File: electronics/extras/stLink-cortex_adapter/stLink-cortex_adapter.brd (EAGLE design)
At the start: 11.4 x 20.3 mm, 2 parts, among them J15 Cortex Debug

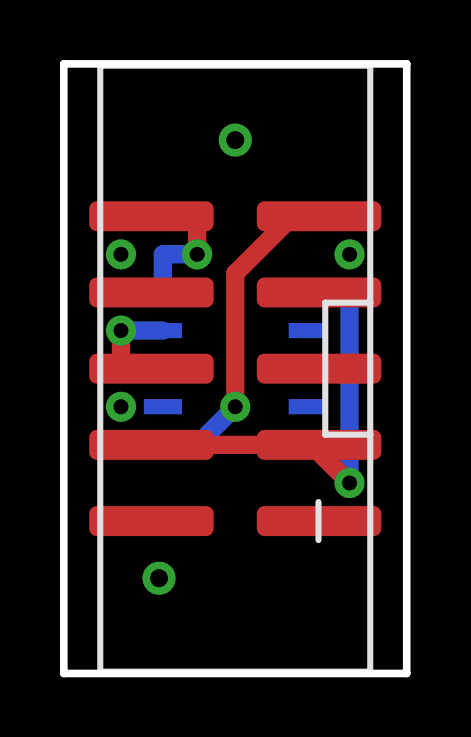
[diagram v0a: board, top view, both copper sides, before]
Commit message: Labwiz T420 module gerbers generated.
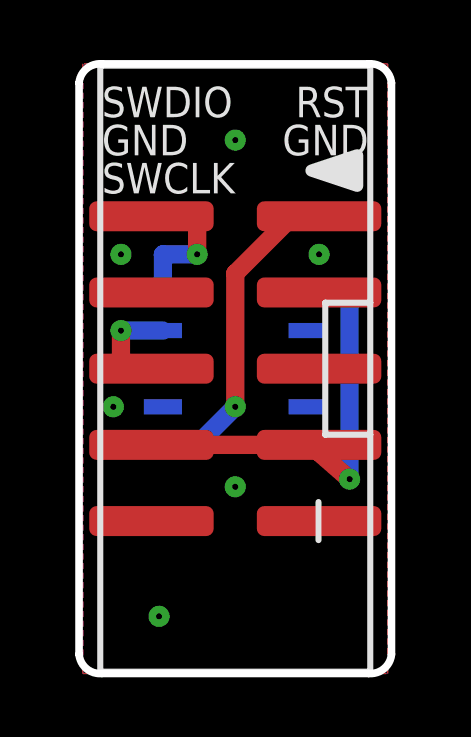
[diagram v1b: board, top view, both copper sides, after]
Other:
- board size 11.4 x 20.3 mm -> 10.4 x 20.3 mm
- board text added: "ST-Linkv2 Cortex"
- board text removed: "ST-Link v2 Cortex Adapter"
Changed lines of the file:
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@@
 <setting verticaltext="up"/>
 </settings>
-<grid distance="0.025" unitdist="inch" unit="inch" style="lines" multiple="1" display="yes" altdistance="0.05" altunitdist="mil" altunit="inch"/>
+<grid distance="5" unitdist="mil" unit="mil" style="lines" multiple="1" display="yes" altdistance="0.05" altunitdist="mil" altunit="inch"/>
 <layers>
 <layer number="1" name="Top" color="4" fill="1" visible="yes" active="yes"/>
@@
 <layer number="49" name="Reference" color="7" fill="1" visible="yes" active="yes"/>
 <layer number="50" name="dxf" color="7" fill="1" visible="no" active="no"/>
-<layer number="51" name="tDocu" color="6" fill="1" visible="yes" active="yes"/>
-<layer number="52" name="bDocu" color="7" fill="1" visible="yes" active="yes"/>
+<layer number="51" name="tDocu" color="6" fill="1" visible="no" active="yes"/>
+<layer number="52" name="bDocu" color="7" fill="1" visible="no" active="yes"/>
 <layer number="53" name="tGND_GNDA" color="7" fill="9" visible="no" active="no"/>
 <layer number="54" name="bGND_GNDA" color="1" fill="9" visible="no" active="no"/>
@@
 <board>
 <plain>
-<wire x1="-0.635" y1="0" x2="-0.635" y2="20.32" width="0.254" layer="20"/>
-<wire x1="-0.635" y1="20.32" x2="10.795" y2="20.32" width="0.254" layer="20"/>
-<wire x1="10.795" y1="20.32" x2="10.795" y2="0" width="0.254" layer="20"/>
-<wire x1="10.795" y1="0" x2="-0.635" y2="0" width="0.254" layer="20"/>
+<wire x1="9.525" y1="0" x2="0.635" y2="0" width="0.254" layer="20"/>
+<wire x1="0.635" y1="0" x2="-0.127" y2="0.635" width="0.254" layer="20" curve="-90"/>
+<wire x1="-0.127" y1="0.635" x2="-0.127" y2="19.685" width="0.254" layer="20"/>
+<wire x1="-0.127" y1="19.685" x2="0.635" y2="20.32" width="0.254" layer="20" curve="-90"/>
+<wire x1="0.635" y1="20.32" x2="9.525" y2="20.32" width="0.254" layer="20"/>
+<wire x1="9.525" y1="20.32" x2="10.287" y2="19.685" width="0.254" layer="20" curve="-90"/>
+<wire x1="10.287" y1="19.685" x2="10.287" y2="0.635" width="0.254" layer="20"/>
+<wire x1="10.287" y1="0.635" x2="9.525" y2="0" width="0.254" layer="20" curve="-90"/>
 <text x="10.16" y="15.24" size="1.016" layer="51" align="center-left">RST</text>
 <text x="0" y="12.7" size="1.016" layer="51" rot="R180" align="center-left">GND</text>
@@
 <text x="0" y="7.62" size="1.016" layer="51" rot="R180" align="center-left">3.3V</text>
 <text x="10.16" y="7.62" size="1.016" layer="51" align="center-left">3.3V</text>
-<text x="0.635" y="19.05" size="1.016" layer="22" rot="MR180" align="center-left">SWDIO</text>
-<text x="0.635" y="17.78" size="1.016" layer="22" rot="MR180" align="center-left">GND</text>
-<text x="0.635" y="16.51" size="1.016" layer="22" rot="MR180" align="center-left">SWCLK</text>
-<text x="0.635" y="15.24" size="1.016" layer="22" rot="MR180" align="center-left">3.3V</text>
-<text x="9.525" y="19.05" size="1.016" layer="22" rot="MR0" align="center-left">RST</text>
-<text x="9.525" y="15.24" size="1.016" layer="22" rot="MR0" align="center-left">3.3V</text>
-<text x="9.525" y="17.78" size="1.016" layer="22" rot="MR0" align="center-left">GND</text>
-<text x="9.525" y="6.35" size="1.4224" layer="22" rot="MR0" align="top-left">ST-Link v2
-Cortex
-Adapter</text>
+<text x="0.635" y="19.05" size="1.016" layer="22" font="vector" rot="MR180" align="center-left">SWDIO</text>
+<text x="0.635" y="17.78" size="1.016" layer="22" font="vector" rot="MR180" align="center-left">GND</text>
+<text x="0.635" y="16.51" size="1.016" layer="22" font="vector" rot="MR180" align="center-left">SWCLK</text>
+<text x="0.635" y="15.24" size="1.016" layer="22" font="vector" rot="MR180" align="center-left">3.3V</text>
+<text x="9.525" y="19.05" size="1.016" layer="22" font="vector" rot="MR0" align="center-left">RST</text>
+<text x="9.525" y="15.24" size="1.016" layer="22" font="vector" rot="MR0" align="center-left">3.3V</text>
+<text x="9.525" y="17.78" size="1.016" layer="22" font="vector" rot="MR0" align="center-left">GND</text>
+<text x="9.525" y="3.81" size="1.143" layer="22" font="vector" rot="MR0" align="top-left">ST-Linkv2
+Cortex</text>
+<polygon width="0.4064" layer="21">
+<vertex x="7.62" y="16.764"/>
+<vertex x="9.144" y="16.256"/>
+<vertex x="9.144" y="17.272"/>
+</polygon>
+<text x="9.525" y="19.05" size="1.016" layer="21" font="vector" rot="R180" align="center-left">RST</text>
+<text x="9.525" y="17.78" size="1.016" layer="21" font="vector" rot="R180" align="center-left">GND</text>
+<text x="0.635" y="19.05" size="1.016" layer="21" font="vector" align="center-left">SWDIO</text>
+<text x="0.635" y="17.78" size="1.016" layer="21" font="vector" align="center-left">GND</text>
+<text x="0.635" y="16.51" size="1.016" layer="21" font="vector" align="center-left">SWCLK</text>
+<polygon width="0.4064" layer="22">
+<vertex x="8.89" y="14.478"/>
+<vertex x="9.398" y="14.478"/>
+<vertex x="9.144" y="13.716"/>
+</polygon>
 </plain>
 <attributes>
@@
 <wire x1="2.286" y1="7.62" x2="7.874" y2="7.62" width="0.6096" layer="1"/>
 <wire x1="7.874" y1="7.62" x2="7.874" y2="7.366" width="0.6096" layer="1"/>
-<wire x1="7.874" y1="7.366" x2="8.89" y2="6.35" width="0.6096" layer="1"/>
-<via x="8.89" y="6.35" extent="1-16" drill="0.5"/>
-<wire x1="8.89" y1="6.35" x2="8.89" y2="12.7" width="0.6096" layer="16"/>
+<wire x1="7.874" y1="7.366" x2="8.89" y2="6.477" width="0.6096" layer="1"/>
+<via x="8.89" y="6.477" extent="1-16" drill="0.2"/>
+<wire x1="8.89" y1="6.477" x2="8.89" y2="12.7" width="0.6096" layer="16"/>
 <wire x1="8.89" y1="12.7" x2="7.493" y2="12.7" width="0.6096" layer="16"/>
 </signal>
@@
 <contactref element="J1" pad="7"/>
 <contactref element="J1" pad="8"/>
-<via x="2.54" y="3.175" extent="1-16" drill="0.6" shape="square"/>
-<via x="5.08" y="17.78" extent="1-16" drill="0.6" shape="square"/>
+<via x="2.54" y="1.905" extent="1-16" drill="0.2" shape="square"/>
+<via x="5.08" y="17.78" extent="1-16" drill="0.2" shape="square"/>
 <polygon width="0.254" layer="1">
-<vertex x="-0.635" y="0"/>
-<vertex x="10.795" y="0"/>
-<vertex x="10.795" y="20.32"/>
-<vertex x="-0.635" y="20.32"/>
+<vertex x="0" y="0"/>
+<vertex x="10.16" y="0"/>
+<vertex x="10.16" y="20.32"/>
+<vertex x="0" y="20.32"/>
 </polygon>
 <polygon width="0.254" layer="16">
-<vertex x="-0.635" y="0"/>
-<vertex x="10.795" y="0"/>
-<vertex x="10.795" y="20.32"/>
-<vertex x="-0.635" y="20.32"/>
+<vertex x="0" y="0"/>
+<vertex x="10.16" y="0"/>
+<vertex x="10.16" y="20.32"/>
+<vertex x="0" y="20.32"/>
 </polygon>
-<via x="8.89" y="13.97" extent="1-16" drill="0.5"/>
-<via x="1.27" y="13.97" extent="1-16" drill="0.5"/>
-<via x="1.27" y="8.89" extent="1-16" drill="0.5"/>
+<via x="7.874" y="13.97" extent="1-16" drill="0.2"/>
+<via x="1.27" y="13.97" extent="1-16" drill="0.2"/>
+<via x="1.016" y="8.89" extent="1-16" drill="0.2"/>
+<via x="5.08" y="6.223" extent="1-16" drill="0.2" shape="square"/>
 </signal>
 <signal name="N$3">
@@
 <wire x1="2.286" y1="15.24" x2="3.81" y2="15.24" width="0.6096" layer="1"/>
 <wire x1="3.81" y1="15.24" x2="3.81" y2="13.97" width="0.6096" layer="1"/>
-<via x="3.81" y="13.97" extent="1-16" drill="0.5"/>
+<via x="3.81" y="13.97" extent="1-16" drill="0.2"/>
 <wire x1="3.81" y1="13.97" x2="2.667" y2="13.97" width="0.6096" layer="16"/>
 <wire x1="2.667" y1="13.97" x2="2.667" y2="12.7" width="0.6096" layer="16"/>
@@
 <contactref element="J15" pad="4"/>
 <wire x1="2.667" y1="11.43" x2="1.27" y2="11.43" width="0.6096" layer="16"/>
-<via x="1.27" y="11.43" extent="1-16" drill="0.5"/>
+<via x="1.27" y="11.43" extent="1-16" drill="0.2"/>
 <wire x1="1.27" y1="11.43" x2="1.27" y2="10.16" width="0.6096" layer="1"/>
 <wire x1="1.27" y1="10.16" x2="2.286" y2="10.16" width="0.6096" layer="1"/>
@@
 <wire x1="6.985" y1="15.24" x2="5.08" y2="13.335" width="0.6096" layer="1"/>
 <wire x1="5.08" y1="13.335" x2="5.08" y2="8.89" width="0.6096" layer="1"/>
-<via x="5.08" y="8.89" extent="1-16" drill="0.5"/>
+<via x="5.08" y="8.89" extent="1-16" drill="0.2"/>
 <wire x1="5.08" y1="8.89" x2="3.81" y2="7.62" width="0.6096" layer="16"/>
 <wire x1="3.81" y1="7.62" x2="2.667" y2="7.62" width="0.6096" layer="16"/>
